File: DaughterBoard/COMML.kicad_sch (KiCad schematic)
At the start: 36 parts, among them J2 705510038, J3 705510038

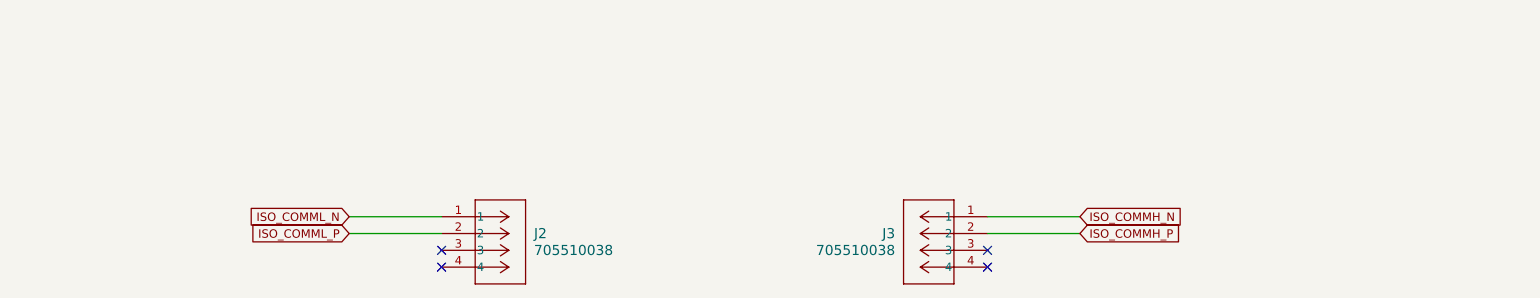
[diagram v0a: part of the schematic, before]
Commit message: m
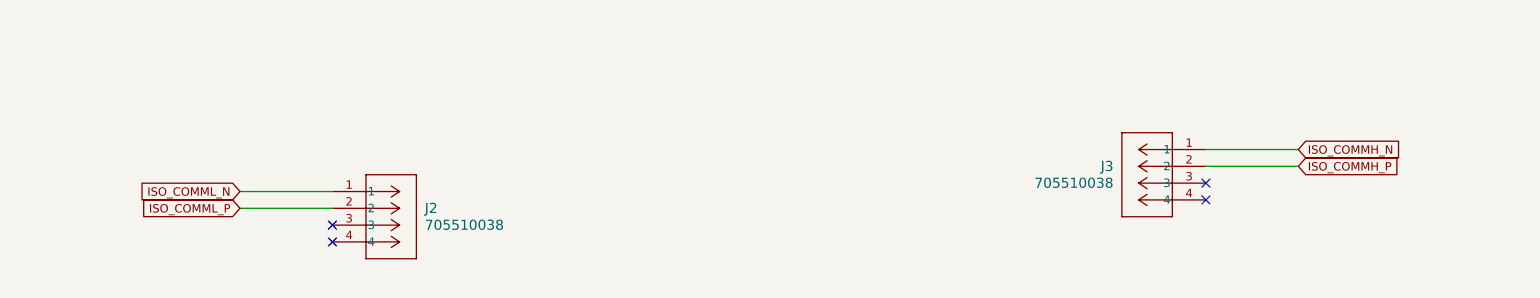
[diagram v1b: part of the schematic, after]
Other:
- moved on the sheet: J2, J3
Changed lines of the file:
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@@
 	)
 	(no_connect
-		(at 154.94 231.14)
+		(at 138.43 227.33)
 	)
 	(no_connect
-		(at 237.49 228.6)
+		(at 270.51 218.44)
 	)
 	(no_connect
-		(at 237.49 231.14)
+		(at 270.51 220.98)
 	)
 	(no_connect
-		(at 154.94 228.6)
+		(at 138.43 224.79)
 	)
 	(wire
@@
 	(wire
 		(pts
-			(xy 140.97 226.06) (xy 154.94 226.06)
+			(xy 124.46 222.25) (xy 138.43 222.25)
 		)
 		(stroke
@@
 	(wire
 		(pts
-			(xy 140.97 223.52) (xy 154.94 223.52)
+			(xy 124.46 219.71) (xy 138.43 219.71)
 		)
 		(stroke
@@
 	(wire
 		(pts
-			(xy 251.46 226.06) (xy 237.49 226.06)
+			(xy 284.48 215.9) (xy 270.51 215.9)
 		)
 		(stroke
@@
 	(wire
 		(pts
-			(xy 251.46 223.52) (xy 237.49 223.52)
+			(xy 284.48 213.36) (xy 270.51 213.36)
 		)
 		(stroke
@@
 	(global_label "ISO_COMMH_N"
 		(shape input)
-		(at 251.46 223.52 0)
+		(at 284.48 213.36 0)
 		(fields_autoplaced yes)
 		(effects
@@
 		)
 		(property "Intersheetrefs" "${INTERSHEET_REFS}"
-			(at 267.6895 223.52 0)
+			(at 300.7095 213.36 0)
 			(effects
 				(font
@@
 	(global_label "ISO_COMML_N"
 		(shape input)
-		(at 140.97 223.52 180)
+		(at 124.46 219.71 180)
 		(fields_autoplaced yes)
 		(effects
@@
 		)
 		(property "Intersheetrefs" "${INTERSHEET_REFS}"
-			(at 125.0429 223.52 0)
+			(at 108.5329 219.71 0)
 			(effects
 				(font
@@
 	(global_label "ISO_COMML_P"
 		(shape input)
-		(at 140.97 226.06 180)
+		(at 124.46 222.25 180)
 		(fields_autoplaced yes)
 		(effects
@@
 		)
 		(property "Intersheetrefs" "${INTERSHEET_REFS}"
-			(at 125.1034 226.06 0)
+			(at 108.5934 222.25 0)
 			(effects
 				(font
@@
 	(global_label "ISO_COMMH_P"
 		(shape input)
-		(at 251.46 226.06 0)
+		(at 284.48 215.9 0)
 		(fields_autoplaced yes)
 		(effects
@@
 		)
 		(property "Intersheetrefs" "${INTERSHEET_REFS}"
-			(at 267.629 226.06 0)
+			(at 300.649 215.9 0)
 			(effects
 				(font
@@
 	(symbol
 		(lib_id "0705510038:705510038")
-		(at 237.49 223.52 0)
+		(at 270.51 213.36 0)
 		(mirror y)
 		(unit 1)
@@
 		(fields_autoplaced yes)
 		(property "Reference" "J3"
-			(at 223.52 226.0599 0)
+			(at 256.54 215.8999 0)
 			(effects
 				(font
@@
 		)
 		(property "Value" "705510038"
-			(at 223.52 228.5999 0)
+			(at 256.54 218.4399 0)
 			(effects
 				(font
@@
 		)
 		(property "Footprint" "CONN_70551-xxxx_04_MOL"
-			(at 237.49 223.52 0)
+			(at 270.51 213.36 0)
 			(effects
 				(font
@@
 		)
 		(property "Datasheet" "705510038"
-			(at 237.49 223.52 0)
+			(at 270.51 213.36 0)
 			(effects
 				(font
@@
 		)
 		(property "Description" ""
-			(at 237.49 223.52 0)
+			(at 270.51 213.36 0)
 			(effects
 				(font
@@
 	(symbol
 		(lib_id "0705510038:705510038")
-		(at 154.94 223.52 0)
+		(at 138.43 219.71 0)
 		(unit 1)
 		(exclude_from_sim no)
@@
 		(fields_autoplaced yes)
 		(property "Reference" "J2"
-			(at 168.91 226.0599 0)
+			(at 152.4 222.2499 0)
 			(effects
 				(font
@@
 		)
 		(property "Value" "705510038"
-			(at 168.91 228.5999 0)
+			(at 152.4 224.7899 0)
 			(effects
 				(font
@@
 		)
 		(property "Footprint" "CONN_70551-xxxx_04_MOL"
-			(at 154.94 223.52 0)
+			(at 138.43 219.71 0)
 			(effects
 				(font
@@
 		)
 		(property "Datasheet" "705510038"
-			(at 154.94 223.52 0)
+			(at 138.43 219.71 0)
 			(effects
 				(font
@@
 		)
 		(property "Description" ""
-			(at 154.94 223.52 0)
-			(effects
-				(font
+			(at 138.43 219.71 0)
+			(effects
+				(font
